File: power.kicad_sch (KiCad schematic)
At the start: 45 parts, among them J13 USB_C_Receptacle_PowerOnly_6P, J14 Conn_01x01, J17 Conn_01x01, J18 Conn_01x01, J19 Conn_01x01, U24 TBA1-0522E, U25 TBA1-0522E, U26 TBA1-0522E

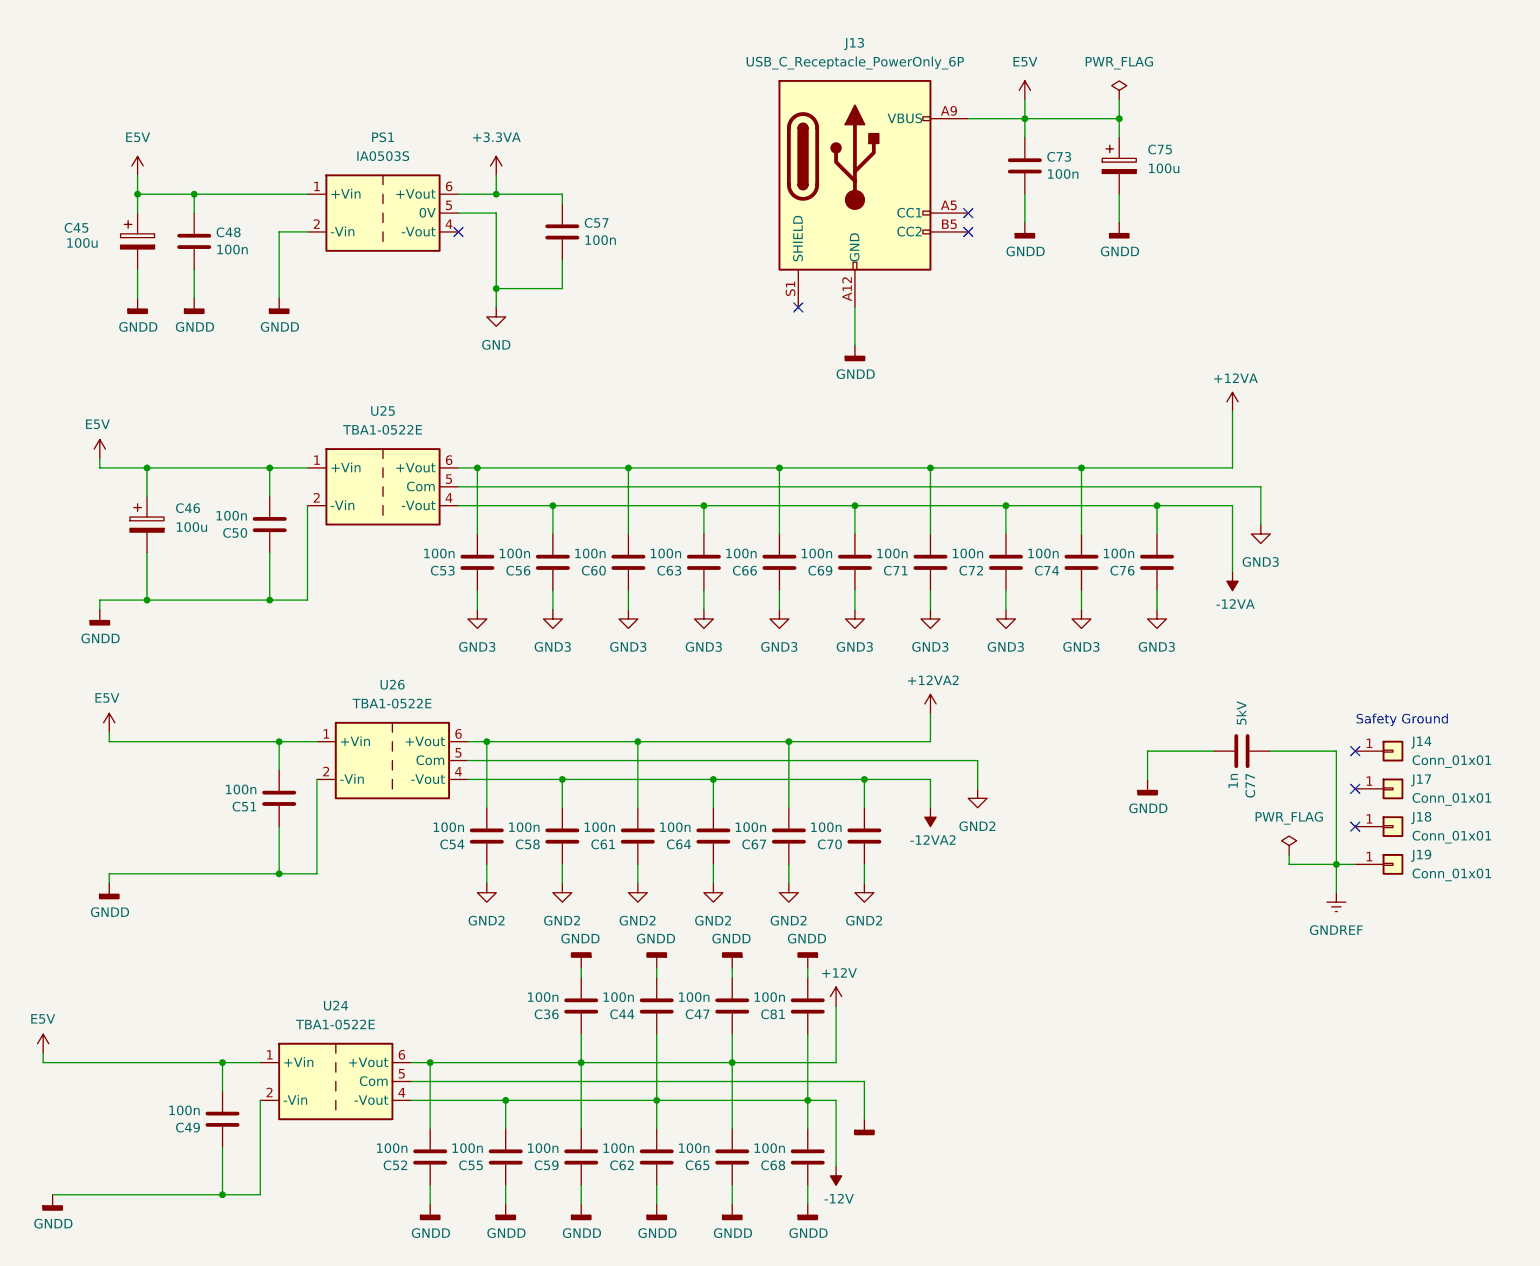
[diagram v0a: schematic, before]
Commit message: alueet laatikoitu, ensimmäiset input osat laitettu
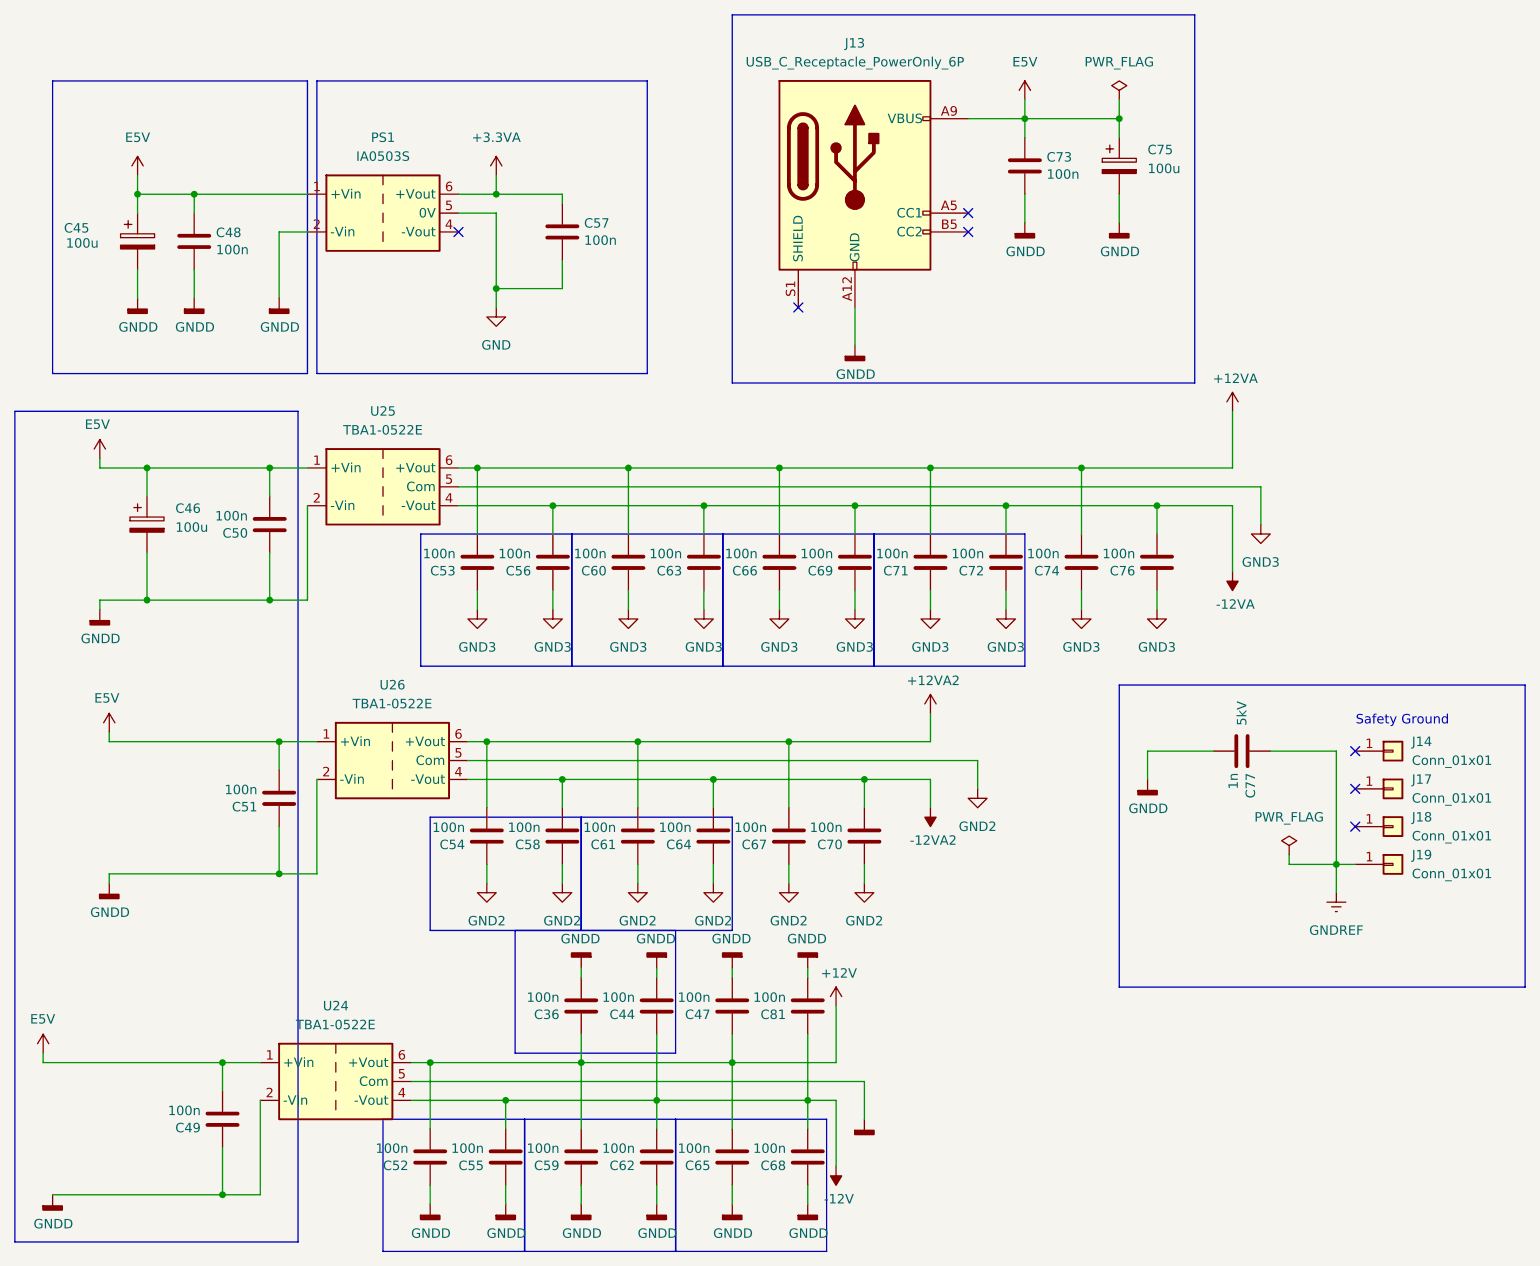
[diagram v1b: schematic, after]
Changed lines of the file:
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@@
 	(generator_version "9.0")
 	(paper "A4")
+	(rectangle
+		(start 97.79 95.25)
+		(end 118.11 113.03)
+		(stroke
+			(width 0)
+			(type default)
+		)
+		(fill
+			(type none)
+		)
+	)
+	(rectangle
+		(start 110.49 148.59)
+		(end 132.08 165.1)
+		(stroke
+			(width 0)
+			(type default)
+		)
+		(fill
+			(type none)
+		)
+	)
+	(rectangle
+		(start 118.11 95.25)
+		(end 138.43 113.03)
+		(stroke
+			(width 0)
+			(type default)
+		)
+		(fill
+			(type none)
+		)
+	)
+	(rectangle
+		(start 92.71 173.99)
+		(end 111.76 191.77)
+		(stroke
+			(width 0)
+			(type default)
+		)
+		(fill
+			(type none)
+		)
+	)
+	(rectangle
+		(start 43.18 78.74)
+		(end 81.28 190.5)
+		(stroke
+			(width 0)
+			(type default)
+			(color 253 1 255 1)
+		)
+		(fill
+			(type none)
+		)
+	)
+	(rectangle
+		(start 48.26 34.29)
+		(end 82.55 73.66)
+		(stroke
+			(width 0)
+			(type default)
+			(color 255 9 241 1)
+		)
+		(fill
+			(type none)
+		)
+	)
+	(rectangle
+		(start 99.06 133.35)
+		(end 119.38 148.59)
+		(stroke
+			(width 0)
+			(type default)
+		)
+		(fill
+			(type none)
+		)
+	)
+	(rectangle
+		(start 111.76 173.99)
+		(end 132.08 191.77)
+		(stroke
+			(width 0)
+			(type default)
+		)
+		(fill
+			(type none)
+		)
+	)
+	(rectangle
+		(start 139.7 25.4)
+		(end 201.93 74.93)
+		(stroke
+			(width 0)
+			(type default)
+			(color 255 9 241 1)
+		)
+		(fill
+			(type none)
+		)
+	)
+	(rectangle
+		(start 138.43 95.25)
+		(end 158.75 113.03)
+		(stroke
+			(width 0)
+			(type default)
+		)
+		(fill
+			(type none)
+		)
+	)
+	(rectangle
+		(start 132.08 173.99)
+		(end 152.4 191.77)
+		(stroke
+			(width 0)
+			(type default)
+		)
+		(fill
+			(type none)
+		)
+	)
+	(rectangle
+		(start 83.82 34.29)
+		(end 128.27 73.66)
+		(stroke
+			(width 0)
+			(type default)
+			(color 250 7 255 1)
+		)
+		(fill
+			(type none)
+		)
+	)
+	(rectangle
+		(start 119.38 133.35)
+		(end 139.7 148.59)
+		(stroke
+			(width 0)
+			(type default)
+		)
+		(fill
+			(type none)
+		)
+	)
+	(rectangle
+		(start 191.77 115.57)
+		(end 246.38 156.21)
+		(stroke
+			(width 0)
+			(type default)
+			(color 255 9 241 1)
+		)
+		(fill
+			(type none)
+		)
+	)
+	(rectangle
+		(start 158.75 95.25)
+		(end 179.07 113.03)
+		(stroke
+			(width 0)
+			(type default)
+		)
+		(fill
+			(type none)
+		)
+	)
 	(text "Safety Ground\n"
 		(exclude_from_sim no)
